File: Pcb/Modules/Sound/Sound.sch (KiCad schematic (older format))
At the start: 15 parts, among them J1 JACK_RJ45, U1 MAX4466

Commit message: Update sound module
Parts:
- C1: value 0.1uF -> 47uF; footprint Capacitors_SMD:C_0603 -> Capacitors_SMD:C_1206
- C2: value 0.01uF -> 1uF
- C3: value 10uF -> 0.1uF; footprint Capacitors_SMD:C_1206 -> Capacitors_SMD:C_0603
- C4: value 100pF -> 47pF
- R2: value 1K -> 2.2K
- R3, R4: value 1M -> 100K
- R5: value 1K -> 20K
- R6: value 100K -> 1M
- U1: footprint TO_SOT_Packages_SMD:SOT-23-5 -> TO_SOT_Packages_SMD:SOT-353_SC-70-5
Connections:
- wire segments 35 -> 38
- no-connect marks 0 -> 6
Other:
- note added: "Gain = (R6/R5)+1 = 51"
- note removed: "Gain = (R6/R5)+1 = 101"
- moved on the sheet: C1, C2, C3, C4, J1, MK1, R1, R2, R3, R4, R5, R6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

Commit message: Update module pcbs
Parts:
- removed L1, L2: Ferrite_Bead, Resistors_SMD:R_0805, symbol Ferrite_Bead
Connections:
- wire segments 38 -> 36
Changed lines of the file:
@@
-$EndComp
-$Comp
-L Ferrite_Bead L2
-U 1 1 59BF0A07
-P 3550 4400
-F 0 "L2" V 3400 4425 50  0000 C CNN
-F 1 "Ferrite_Bead" V 3700 4400 50  0000 C CNN
-F 2 "Resistors_SMD:R_0805" V 3480 4400 50  0001 C CNN
-F 3 "" H 3550 4400 50  0000 C CNN
-	1    3550 4400
-	0    1    1    0
 $EndComp
 $Comp
@@
 AN_VAL
 $Comp
-L Ferrite_Bead L1
-U 1 1 59C00684
-P 2150 4400
-F 0 "L1" V 2000 4425 50  0000 C CNN
-F 1 "Ferrite_Bead" V 2300 4400 50  0000 C CNN
-F 2 "Resistors_SMD:R_0805" V 2080 4400 50  0001 C CNN
-F 3 "" H 2150 4400 50  0000 C CNN
-	1    2150 4400
-	0    1    1    0
-$EndComp
-$Comp
 L GND #PWR07
 U 1 1 59C00872
@@
 Connection ~ 4200 1850
 Wire Wire Line
-	3400 4400 3200 4400
+	3200 4400 3850 4400
 Wire Wire Line
 	3200 4400 3200 4550
 Wire Wire Line
-	2500 4550 2500 4400
-Wire Wire Line
-	2500 4400 2300 4400
-Wire Wire Line
-	2000 4400 1850 4400
+	2500 4400 2500 4550
+Wire Wire Line
+	1850 4400 2500 4400
 Wire Wire Line
 	1850 4400 1850 4600
 Wire Wire Line
-	3700 4400 3850 4400
-Wire Wire Line
 	3100 4550 3100 4250

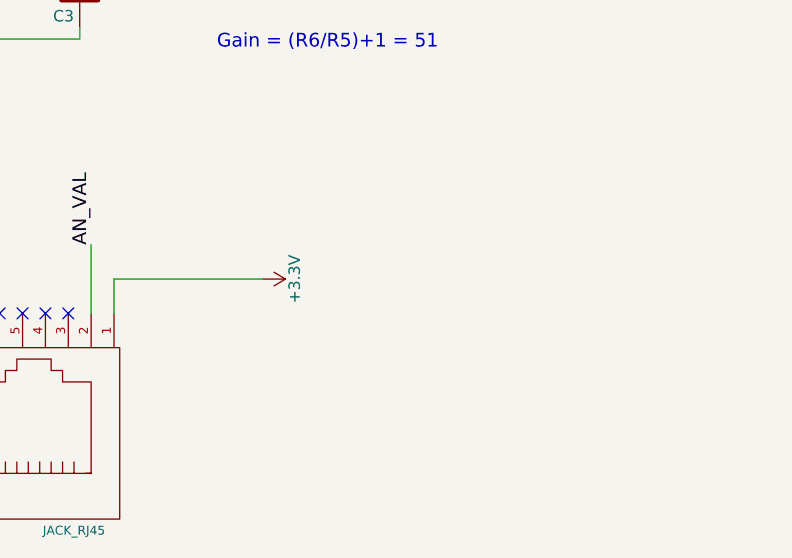
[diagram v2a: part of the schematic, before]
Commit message: Update PCBs
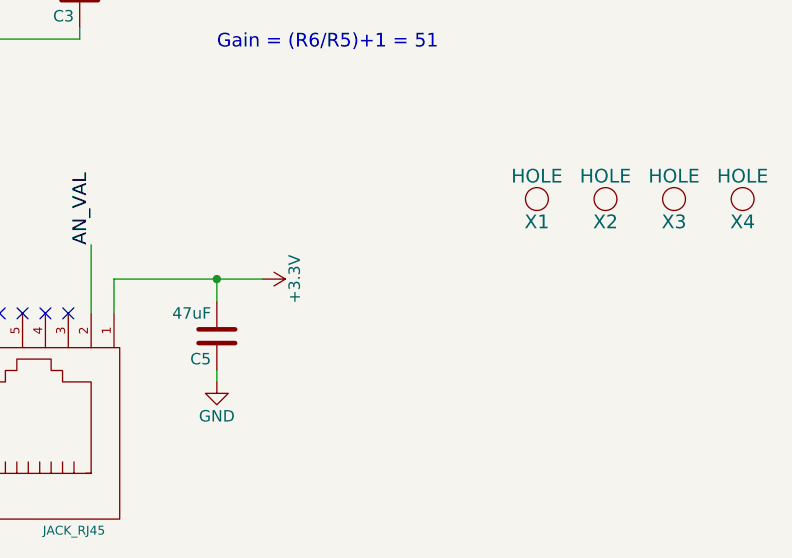
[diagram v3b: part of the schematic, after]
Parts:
- added C5: 47uF, Capacitors_SMD:C_1206, symbol C
- added X1, X2, X3, X4: HOLE, Mounting_Holes:MountingHole_2.5mm_Pad, symbol HOLE
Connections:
- net +3V3: now also C5.2
- net GND: now also C5.1
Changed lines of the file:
@@
 NoConn ~ 2600 4550
 NoConn ~ 6050 2750
+$Comp
+L HOLE X1
+U 1 1 5A23D852
+P 5050 4050
+F 0 "X1" H 5050 3950 60  0000 C CNN
+F 1 "HOLE" H 5050 4150 60  0000 C CNN
+F 2 "Mounting_Holes:MountingHole_2.5mm_Pad" H 5050 4050 60  0001 C CNN
+F 3 "" H 5050 4050 60  0000 C CNN
+	1    5050 4050
+	1    0    0    -1
+$EndComp
+$Comp
+L HOLE X2
+U 1 1 5A23DBBB
+P 5350 4050
+F 0 "X2" H 5350 3950 60  0000 C CNN
+F 1 "HOLE" H 5350 4150 60  0000 C CNN
+F 2 "Mounting_Holes:MountingHole_2.5mm_Pad" H 5350 4050 60  0001 C CNN
+F 3 "" H 5350 4050 60  0000 C CNN
+	1    5350 4050
+	1    0    0    -1
+$EndComp
+$Comp
+L HOLE X3
+U 1 1 5A23DC00
+P 5650 4050
+F 0 "X3" H 5650 3950 60  0000 C CNN
+F 1 "HOLE" H 5650 4150 60  0000 C CNN
+F 2 "Mounting_Holes:MountingHole_2.5mm_Pad" H 5650 4050 60  0001 C CNN
+F 3 "" H 5650 4050 60  0000 C CNN
+	1    5650 4050
+	1    0    0    -1
+$EndComp
+$Comp
+L HOLE X4
+U 1 1 5A23DC48
+P 5950 4050
+F 0 "X4" H 5950 3950 60  0000 C CNN
+F 1 "HOLE" H 5950 4150 60  0000 C CNN
+F 2 "Mounting_Holes:MountingHole_2.5mm_Pad" H 5950 4050 60  0001 C CNN
+F 3 "" H 5950 4050 60  0000 C CNN
+	1    5950 4050
+	1    0    0    -1
+$EndComp
+$Comp
+L C C5
+U 1 1 5A241B9D
+P 3650 4650
+F 0 "C5" H 3675 4750 50  0000 L CNN
+F 1 "47uF" H 3675 4550 50  0000 L CNN
+F 2 "Capacitors_SMD:C_1206" H 3688 4500 50  0001 C CNN
+F 3 "" H 3650 4650 50  0000 C CNN
+	1    3650 4650
+	-1   0    0    1
+$EndComp
+$Comp
+L GND #PWR010
+U 1 1 5A241E23
+P 3650 4850
+F 0 "#PWR010" H 3650 4600 50  0001 C CNN
+F 1 "GND" H 3650 4700 50  0000 C CNN
+F 2 "" H 3650 4850 50  0000 C CNN
+F 3 "" H 3650 4850 50  0000 C CNN
+	1    3650 4850
+	1    0    0    -1
+$EndComp
+Wire Wire Line
+	3650 4850 3650 4800
+Wire Wire Line
+	3650 4500 3650 4400
+Connection ~ 3650 4400
 $EndSCHEMATC

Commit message: Update pcb for new switch
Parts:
- C1, C2, C3, C4, C5: symbol C -> Device:C
- J1: symbol JACK_RJ45 -> CA6:JACK_RJ45
- MK1: symbol Microphone_Condenser -> Device:Microphone_Condenser
- R1, R2, R3, R4, R5, R6: symbol R -> Device:R
- U1: symbol OPA376AIDCK -> Sound-rescue:OPA376AIDCK
- X1, X2, X3, X4: symbol HOLE -> CA6:HOLE
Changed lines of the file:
@@
-EESchema Schematic File Version 2
-LIBS:power
-LIBS:device
-LIBS:transistors
-LIBS:conn
-LIBS:linear
-LIBS:regul
-LIBS:74xx
-LIBS:cmos4000
-LIBS:adc-dac
-LIBS:memory
-LIBS:xilinx
-LIBS:microcontrollers
-LIBS:dsp
-LIBS:microchip
-LIBS:analog_switches
-LIBS:motorola
-LIBS:texas
-LIBS:intel
-LIBS:audio
-LIBS:interface
-LIBS:digital-audio
-LIBS:philips
-LIBS:display
-LIBS:cypress
-LIBS:siliconi
-LIBS:opto
-LIBS:atmel
-LIBS:contrib
-LIBS:valves
-LIBS:CA6
+EESchema Schematic File Version 4
 LIBS:Sound-cache
-EELAYER 25 0
+EELAYER 26 0
 EELAYER END
 $Descr A4 11693 8268
@@
 $EndDescr
 $Comp
-L OPA376AIDCK U1
+L Sound-rescue:OPA376AIDCK U1
 U 1 1 59BF073B
 P 3650 1850
@@
 $EndComp
 $Comp
-L Microphone_Condenser MK1
+L Device:Microphone_Condenser MK1
 U 1 1 59BF08F8
 P 1350 3600
@@
 $EndComp
 $Comp
-L R R1
+L Device:R R1
 U 1 1 59BF092D
 P 1750 2400
@@
 $EndComp
 $Comp
-L C C1
+L Device:C C1
 U 1 1 59BF0968
 P 2050 2800
@@
 $EndComp
 $Comp
-L JACK_RJ45 J1
+L CA6:JACK_RJ45 J1
 U 1 1 59BF1311
 P 2850 5000
@@
 $EndComp
 $Comp
-L R R2
+L Device:R R2
 U 1 1 59BFD37D
 P 1750 3150
@@
 $EndComp
 $Comp
-L GND #PWR01
+L power:GND #PWR01
 U 1 1 59BFD42E
 P 2050 3050
@@
 $EndComp
 $Comp
-L +3.3V #PWR02
+L power:+3.3V #PWR02
 U 1 1 59BFD6E2
 P 1750 2150
@@
 $EndComp
 $Comp
-L GND #PWR03
+L power:GND #PWR03
 U 1 1 59BFDB2D
 P 1350 3850
@@
 $EndComp
 $Comp
-L R R3
+L Device:R R3
 U 1 1 59BFE43A
 P 2700 1550
@@
 $EndComp
 $Comp
-L R R4
+L Device:R R4
 U 1 1 59BFE510
 P 2700 1950
@@
 $EndComp
 $Comp
-L +3.3V #PWR04
+L power:+3.3V #PWR04
 U 1 1 59BFED19
 P 2700 1300
@@
 $EndComp
 $Comp
-L GND #PWR05
+L power:GND #PWR05
 U 1 1 59BFED42
 P 2700 2200
@@
 $EndComp
 $Comp
-L C C3
+L Device:C C3
 U 1 1 59BFEF22
 P 3050 3150
@@
 $EndComp
 $Comp
-L GND #PWR06
+L power:GND #PWR06
 U 1 1 59BFF023
 P 3550 2250
@@
 $EndComp
 $Comp
-L C C4
+L Device:C C4
 U 1 1 59BFF149
 P 3550 3000
@@
 $EndComp
 $Comp
-L R R5
+L Device:R R5
 U 1 1 59BFF2B5
 P 3050 2750
@@
 $EndComp
 $Comp
-L R R6
+L Device:R R6
 U 1 1 59BFF4E5
 P 3550 2550
@@
 AN_VAL
 $Comp
-L GND #PWR07
+L power:GND #PWR07
 U 1 1 59C00872
 P 1850 4600
@@
 $EndComp
 $Comp
-L +3.3V #PWR08
+L power:+3.3V #PWR08
 U 1 1 59C009A9
 P 3850 4400
@@
 Gain = (R6/R5)+1 = 51
 $Comp
-L +3.3V #PWR09
+L power:+3.3V #PWR09
 U 1 1 59C0230A
 P 3550 1450
@@
 $EndComp
 $Comp
-L C C2
+L Device:C C2
 U 1 1 59BFDB54
 P 2500 1950
@@
 	1750 2150 1750 2250
 Wire Wire Line
-	1750 2550 1750 3000
+	1750 2550 1750 2600
 Wire Wire Line
 	1750 2600 2050 2600
@@
 Connection ~ 1750 2600
 Wire Wire Line
-	2700 1700 2700 1800
+	2700 1700 2700 1750
 Connection ~ 2700 1750
 Wire Wire Line
-	2700 2100 2700 2200
+	2700 2100 2700 2150
 Wire Wire Line
 	2700 1400 2700 1300
@@
 	3550 2150 3550 2250
 Wire Wire Line
-	3050 2550 3400 2550
+	3050 2550 3250 2550
 Connection ~ 3050 2550
 Wire Wire Line
-	3950 1850 4550 1850
+	3950 1850 4200 1850
 Wire Wire Line
 	4200 2550 4200 1850
 Wire Wire Line
-	3700 2550 4200 2550
+	3700 2550 3900 2550
 Wire Wire Line
 	3250 2550 3250 3000
@@
 Connection ~ 4200 1850
 Wire Wire Line
-	3200 4400 3850 4400
+	3200 4400 3650 4400
 Wire Wire Line
 	3200 4400 3200 4550
@@
 	3350 1950 3050 1950
 Wire Wire Line
-	3050 1950 3050 2600
+	3050 1950 3050 2550
 Wire Wire Line
 	3550 1550 3550 1450
 Wire Wire Line
-	2500 1750 3350 1750
+	2500 1750 2700 1750
 Wire Wire Line
 	2500 1800 2500 1750
@@
 Connection ~ 2700 2150
 Wire Wire Line
-	1350 3350 3050 3350
+	1350 3350 1750 3350
 Wire Wire Line
 	3050 3350 3050 3300
@@
 NoConn ~ 6050 2750
 $Comp
-L HOLE X1
+L CA6:HOLE X1
 U 1 1 5A23D852
 P 5050 4050
@@
 $EndComp
 $Comp
-L HOLE X2
+L CA6:HOLE X2
 U 1 1 5A23DBBB
 P 5350 4050
@@
 $EndComp
 $Comp
-L HOLE X3
+L CA6:HOLE X3
 U 1 1 5A23DC00
 P 5650 4050
@@
 $EndComp
 $Comp
-L HOLE X4
+L CA6:HOLE X4
 U 1 1 5A23DC48
 P 5950 4050
@@
 $EndComp
 $Comp
-L C C5
+L Device:C C5
 U 1 1 5A241B9D
 P 3650 4650
@@
 $EndComp
 $Comp
-L GND #PWR010
+L power:GND #PWR010
 U 1 1 5A241E23
 P 3650 4850
@@
 	3650 4500 3650 4400
 Connection ~ 3650 4400
+Wire Wire Line
+	1750 3350 3050 3350
+Wire Wire Line
+	1750 2600 1750 3000
+Wire Wire Line
+	2700 1750 2700 1800
+Wire Wire Line
+	2700 1750 3350 1750
+Wire Wire Line
+	3050 2550 3050 2600
+Wire Wire Line
+	3250 2550 3400 2550
+Wire Wire Line
+	3900 2550 4200 2550
+Wire Wire Line
+	4200 1850 4550 1850
+Wire Wire Line
+	2700 2150 2700 2200
+Wire Wire Line
+	3650 4400 3850 4400
 $EndSCHEMATC
